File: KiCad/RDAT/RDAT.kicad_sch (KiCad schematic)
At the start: 17 parts

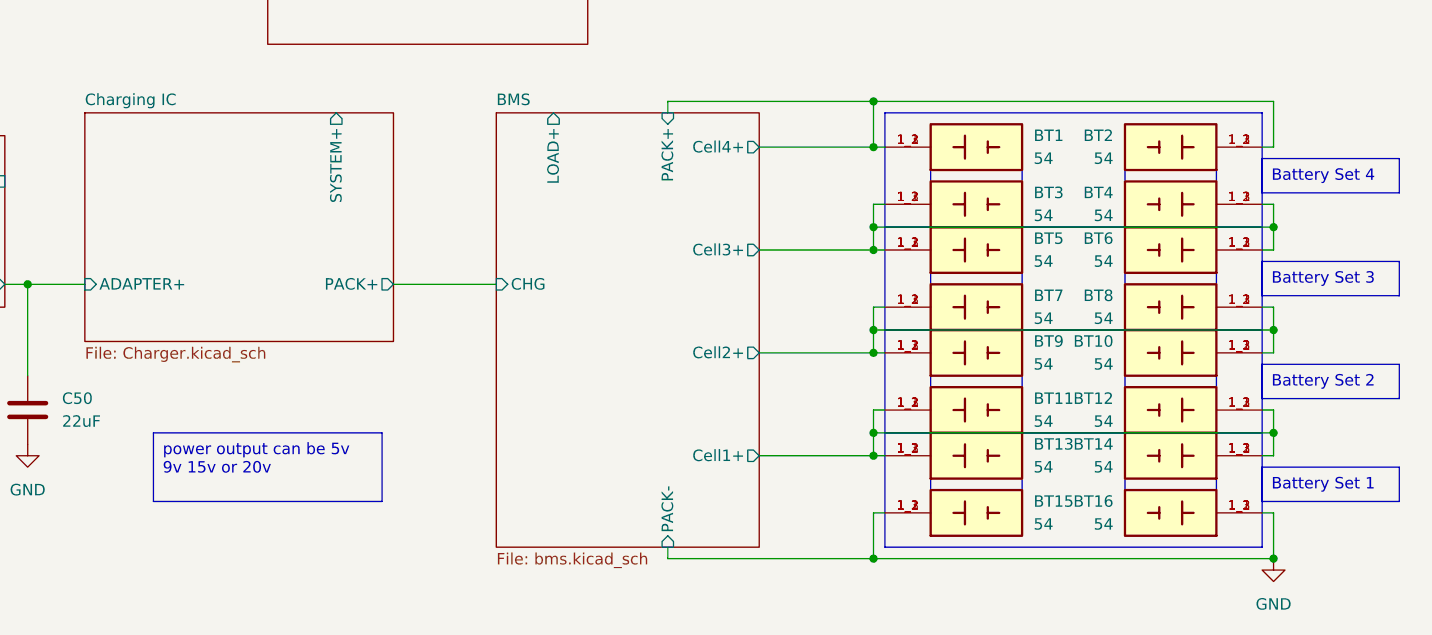
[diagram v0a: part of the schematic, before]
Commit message: added volage stuffs
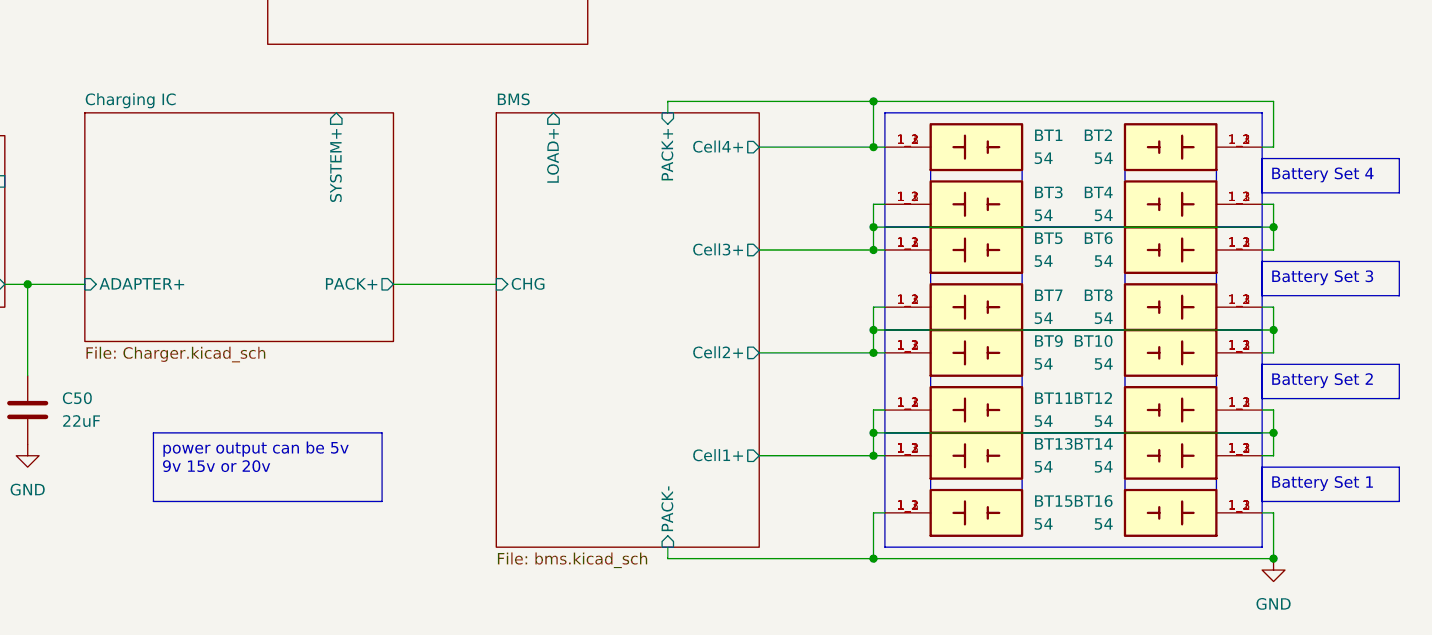
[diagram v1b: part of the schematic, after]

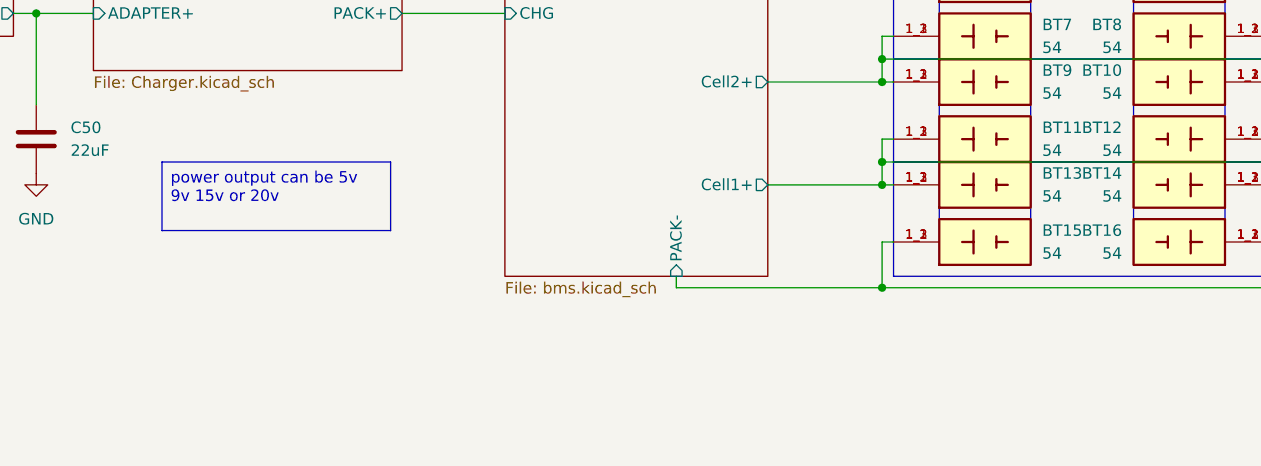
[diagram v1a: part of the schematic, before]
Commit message: Update VRM stuff
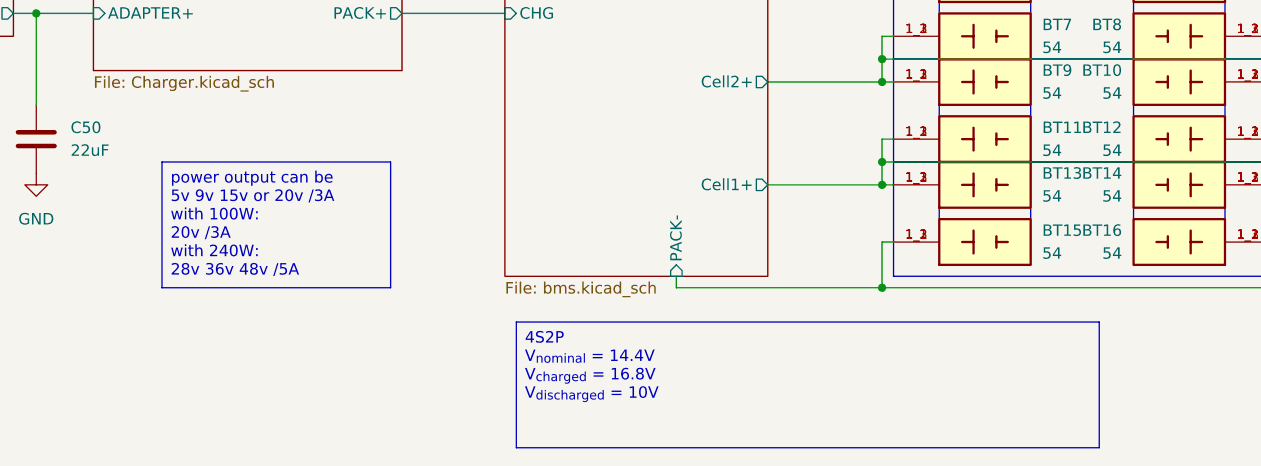
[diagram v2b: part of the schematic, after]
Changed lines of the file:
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@@
 		)
 	)
-	(text_box "power output can be 5v 9v 15v or 20v"
+	(text_box "4S2P\nV_{nominal} = 14.4V\nV_{charged} = 16.8V\nV_{discharged} = 10V"
 		(exclude_from_sim no)
-		(at 60.96 153.67 0)
-		(size 25.4 7.62)
+		(at 100.33 171.45 0)
+		(size 64.77 13.97)
 		(margins 0.9525 0.9525 0.9525 0.9525)
 		(stroke
 			(width 0)
-			(type default)
+			(type solid)
 		)
 		(fill
+			(type none)
+		)
+		(effects
+			(font
+				(size 1.27 1.27)
+			)
+			(justify left top)
+		)
+	)
+	(text_box "power output can be \n5v 9v 15v or 20v /3A\nwith 100W:\n20v /3A\nwith 240W:\n28v 36v 48v /5A"
+		(exclude_from_sim no)
+		(at 60.96 153.67 0)
+		(size 25.4 13.97)
+		(margins 0.9525 0.9525 0.9525 0.9525)
+		(stroke
+			(width 0)
+			(type solid)
+		)
+		(fill
